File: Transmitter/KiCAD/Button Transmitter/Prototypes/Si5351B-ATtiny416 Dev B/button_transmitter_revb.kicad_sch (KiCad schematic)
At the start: 37 parts, among them J1 Antenna Spring, J2 1.27mm Pogo Pads For Programm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, Q1 DMN601TK-7, U101 TPP361081, U102 MIC2288YML, U2 Si5351B-B-GM1, U3 ATtiny416-M, U4 Case, Y1 25MHz

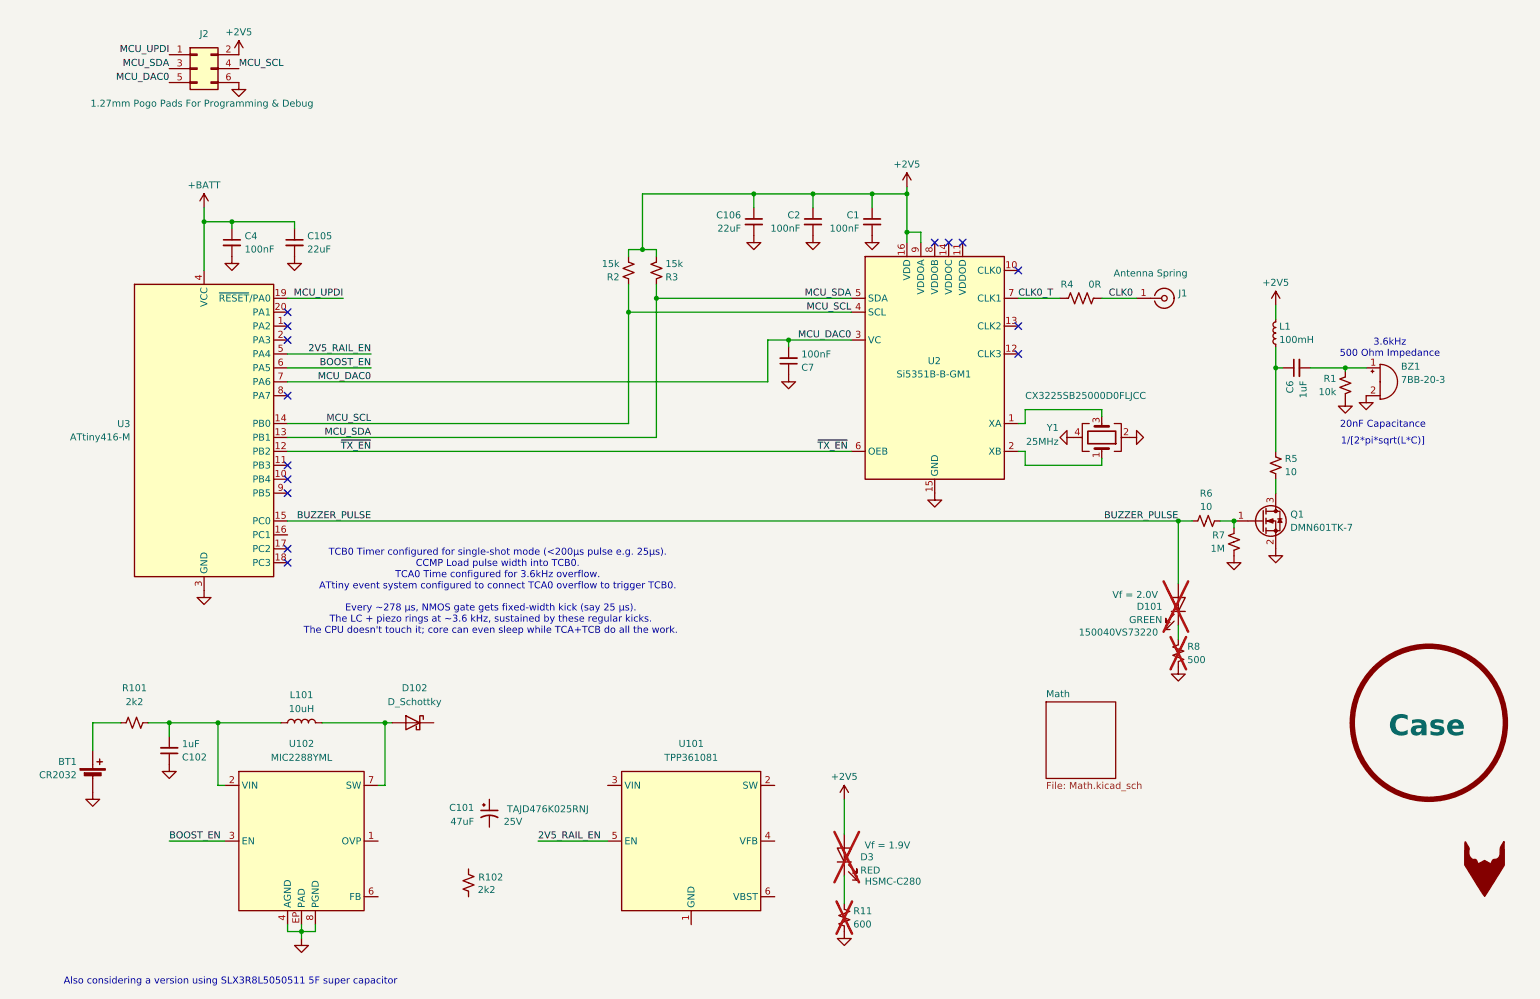
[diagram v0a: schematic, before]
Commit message: Dev 2 Schematic work
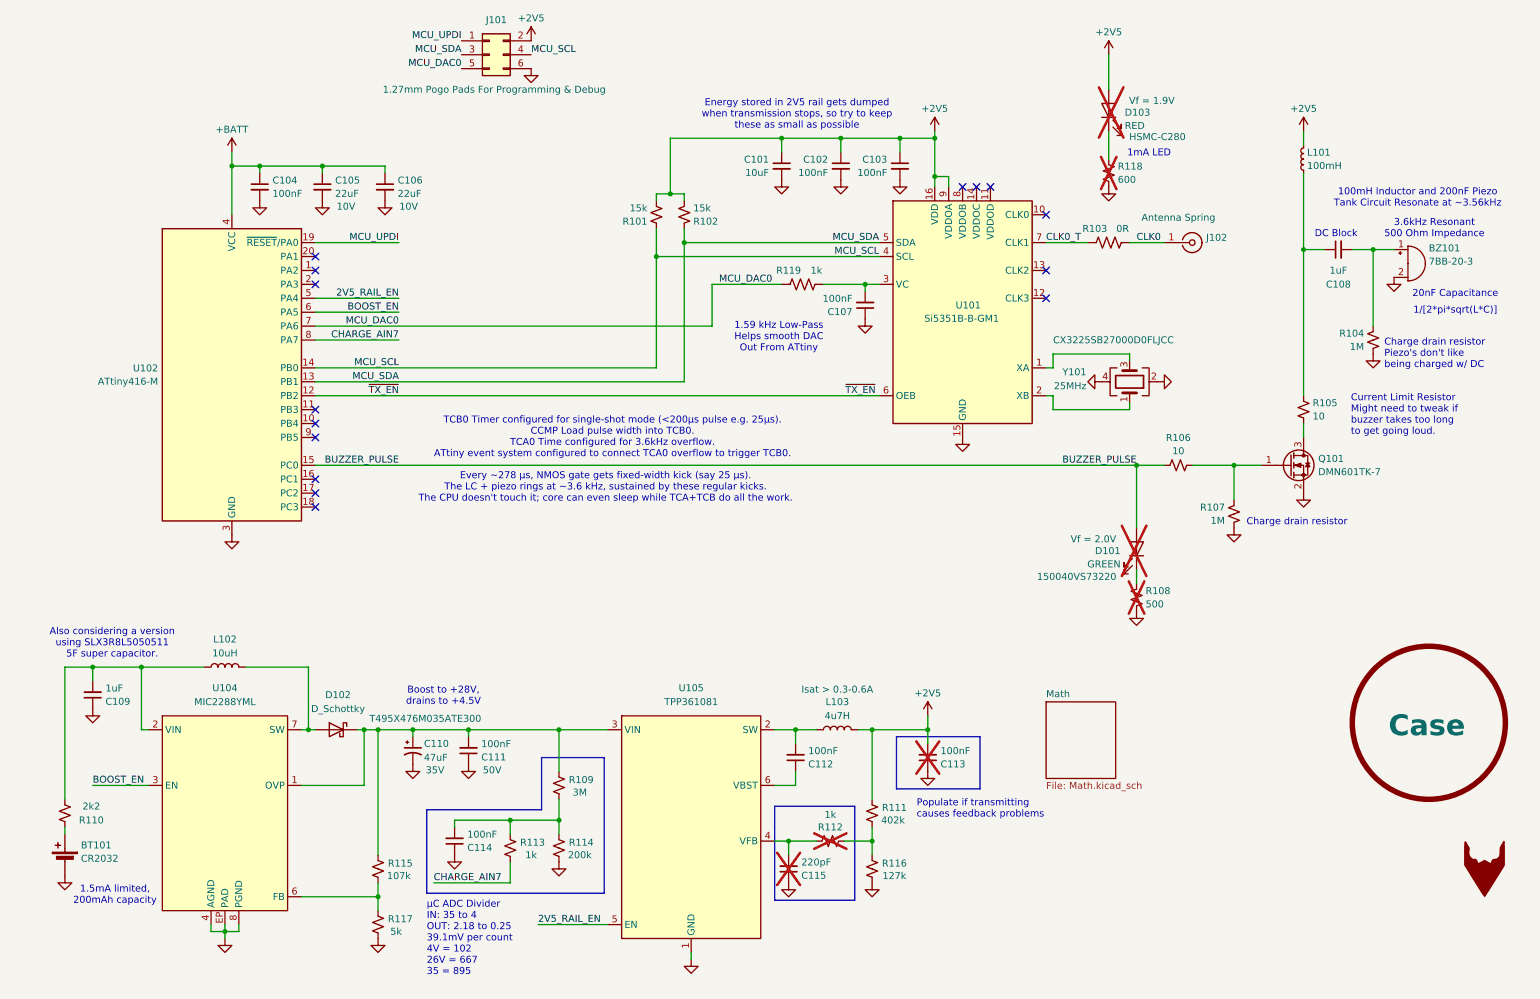
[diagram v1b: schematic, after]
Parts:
- removed C6: 1uF, Library:Worthington_C_0402_1005Metric, symbol Device:C_Small
- added C106: 22uF, Library:Worthington_C_0603_1005Metric, symbol Device:C_Small
- added C108: 1uF, Library:Worthington_C_0402_1005Metric, symbol Device:C_Small
- added C111, C112, C113, C114: 100nF, Library:Worthington_C_0402_1005Metric, symbol Device:C_Small
- added C115: 220pF, Library:Worthington_C_0402_1005Metric, symbol Device:C_Small
- added L103: 4u7H, Library:Worthington_L_0603, symbol Device:L
- added R109: 3M, Library:Worthington_R_0402_1005Metric, symbol Device:R_Small_US
- added R111: 402k, Library:Worthington_R_0402_1005Metric, symbol Device:R_Small_US
- added R112, R113: 1k, Library:Worthington_R_0402_1005Metric, symbol Device:R_Small_US
- added R114: 200k, Library:Worthington_R_0402_1005Metric, symbol Device:R_Small_US
- added R115: 107k, Library:Worthington_R_0402_1005Metric, symbol Device:R_Small_US
- added R116: 127k, Library:Worthington_R_0402_1005Metric, symbol Device:R_Small_US
- added R119: 1k, Library:Worthington_R_0402_1005Metric, symbol Device:R_US
- C101: renamed from C106; value 22uF -> 10uF
- C105: Voltage (none) -> 10V
- C110: renamed from C101; footprint Capacitor_SMD:C_1206_3216Metric -> Library:Worthington_CTant_2917; DigiKey Part TAJD476K025RNJ -> T495X476M035ATE300; Voltage 25V -> 35V
- R104: renamed from R1; value 10k -> 1M
- R117: renamed from R102; value 2k2 -> 5k
- Y101: renamed from Y1; DigiKey (none) -> CX3225SB27000D0FLJCC; Digikey Link (none) -> https://www.digikey.com/en/products/detail/kyocera-avx/CX32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; Field4 CX3225SB25000D0FLJCC -> (none)
- renumbered BT1 to BT101, BZ1 to BZ101, BZ2-1 to BZ2-101, C2 to C102, C1 to C103, C4 to C104, C7 to C107, C102 to C109, D3 to D103, J2 to J101, J1 to J102, L1 to L101, L101 to L102, Q1 to Q101, R2 to R101, R3 to R102, R4 to R103, R5 to R105, R6 to R106, R7 to R107, R8 to R108, R101 to R110, R11 to R118, U2 to U101, U3 to U102, U4 to U103, U102 to U104, U101 to U105
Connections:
- net +2V5: now also C113.2, L103.2, R111.2
- net +BATT: now also C106.1
- net GND: now also C110.2, R117.1, U105.1 (GND), C106.2, C111.1, C113.1, C114.1, C115.1, R114.1, R116.1
- net MCU_DAC0: now also R119.1; no longer C107.2, U101.3 (VC)
- net at L101.1, R105.2: now also C108.1
- net at BZ101.1 (+), R104.1: now also C108.2
- net at R117.2: now also U104.6 (FB), R115.1
- net at U104.1 (OVP): now also C110.1, D102.1 (K), U105.3 (VIN), C111.2, R109.2, R115.2
- net at C109.2, L102.1, U104.2 (VIN): now also R110.1; no longer R110.2
- net at BT101.1 (+): now also R110.2; no longer R110.1
- net CHARGE_AIN7: now reaches U102.8 (PA7)
- net CHARGE_AIN7: now also R113.1
- net at U105.2 (SW): now also C112.2, L103.1
- net at U105.4 (VFB): now also C115.2, R112.2
- net at U105.6 (VBST): now also C112.1
- new net: C114.2, R109.1, R113.2, R114.2
- new net: R111.1, R112.1, R116.2
- new net: C107.2, R119.2, U101.3 (VC)
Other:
- note added: "1.59 kHz Low-Pass Helps smooth DAC Out From ATtiny"
- note added: "1.5mA limited, 200mAh capacity"
- note added: "100mH Inductor and 200nF Piezo Tank Circuit Resonate at ~3.56kHz"
- note added: "1mA LED"
- note added: "3.6kHz Resonant 500 Ohm Impedance"
- note added: "Also considering a version using SLX3R8L5050511 5F super capacitor."
- note added: "Boost to +28V, drains to +4.5V"
- note added: "Charge drain resistor"
- note added: "Charge drain resistor Piezo's don't like being charged w/ DC"
- note added: "Current Limit Resistor Might need to tweak if buzzer takes too long to get going loud."
- note added: "DC Block"
- note added: "Energy stored in 2V5 rail gets dumped when transmission stops, so try to keep these as small as possible"
- note added: "Populate if transmitting causes feedback problems"
- note added: "μC ADC Divider IN: 35 to 4 OUT: 2.18 to 0.25 39.1mV per count 4V = 102 26V = 667 35 = 895"
- note removed: "3.6kHz 500 Ohm Impedance"
- note removed: "Also considering a version using SLX3R8L5050511 5F super capacitor"
- moved on the sheet: BT101, BZ101, C101, C102, C103, C104, C107, C109, C110, D101, D102, D103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
